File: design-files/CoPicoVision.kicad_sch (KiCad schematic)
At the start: 31 parts, among them J101 USB_C_Receptacle_PowerOnly_6P, Q101 MMFTP3334K-AQ, SW101 SW_Push, SW102 SW_Push, U101 Z80CPU, U102 DS1813, U103 74ACT05, U104 ICL7660A, U105 MAX16054, X101 3.579545MHZ

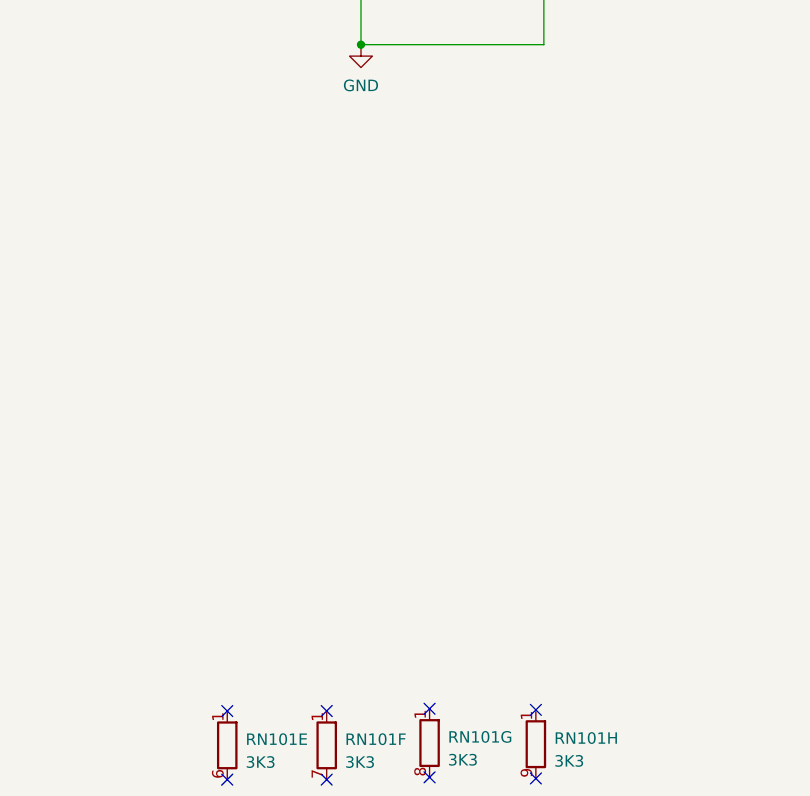
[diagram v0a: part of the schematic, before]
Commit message: Add cartridge connector.
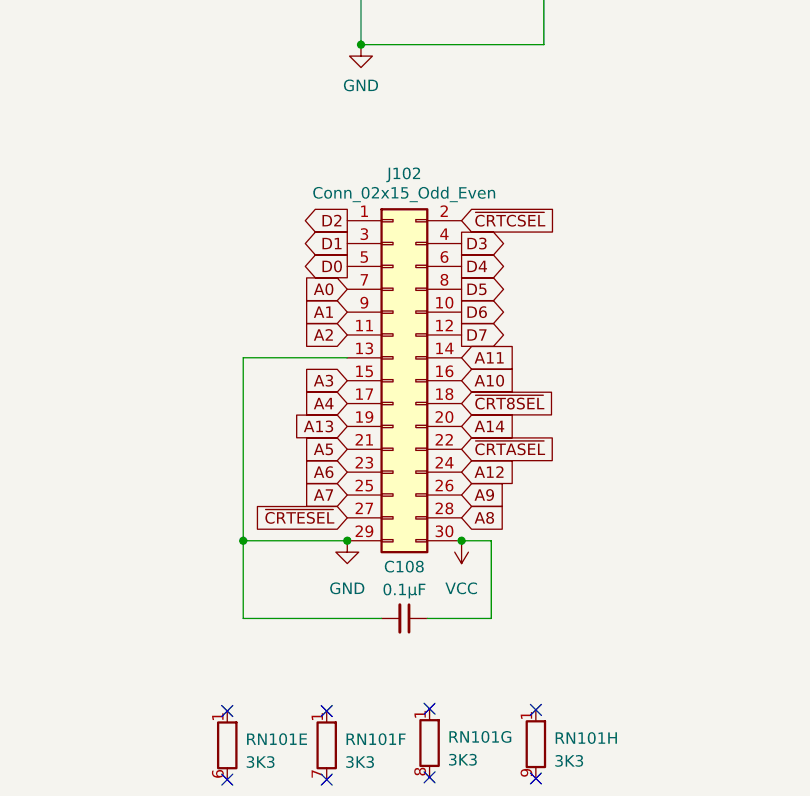
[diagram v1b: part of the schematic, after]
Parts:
- added C108: 0.1µF, Capacitor_SMD:C_0805_2012Metric_Pad1.18x1.45mm_HandSolder, symbol Device:C_Small
- added J102: Conn_02x15_Odd_Even, symbol Connector_Generic:Conn_02x15_Odd_Even
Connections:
- net A0: now also J102.7 (Pin_7)
- net A1: now also J102.9 (Pin_9)
- net A10: now also J102.16 (Pin_16)
- net A11: now also J102.14 (Pin_14)
- net A12: now also J102.24 (Pin_24)
- net A13: now also J102.19 (Pin_19)
- net A14: now also J102.20 (Pin_20)
- net A2: now also J102.11 (Pin_11)
- net A3: now also J102.15 (Pin_15)
- net A4: now also J102.17 (Pin_17)
- net A5: now also J102.21 (Pin_21)
- net A6: now also J102.23 (Pin_23)
- net A7: now also J102.25 (Pin_25)
- net A8: now also J102.28 (Pin_28)
- net A9: now also J102.26 (Pin_26)
- net D0: now also J102.5 (Pin_5)
- net D1: now also J102.3 (Pin_3)
- net D2: now also J102.1 (Pin_1)
- net D3: now also J102.4 (Pin_4)
- net D4: now also J102.6 (Pin_6)
- net D5: now also J102.8 (Pin_8)
- net D6: now also J102.10 (Pin_10)
- net D7: now also J102.12 (Pin_12)
- net GND: now also C108.2, J102.13 (Pin_13), J102.29 (Pin_29)
- net VCC: now also C108.1, J102.30 (Pin_30)
- new net ~{CRT8SEL}: J102.18 (Pin_18)
- new net ~{CRTASEL}: J102.22 (Pin_22)
- new net ~{CRTCSEL}: J102.2 (Pin_2)
- new net ~{CRTESEL}: J102.27 (Pin_27)

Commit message: Cartridge slot.
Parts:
- J102: footprint (none) -> jrt-Connectors:Sullins_Cart_Slot; Mouser (none) -> 571-5530843-2
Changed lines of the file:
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@@
       (effects (font (size 1.27 1.27)))
     )
-    (property "Footprint" "" (at 197.612 117.856 0)
+    (property "Footprint" "jrt-Connectors:Sullins_Cart_Slot" (at 197.612 117.856 0)
       (effects (font (size 1.27 1.27)) hide)
     )
-    (property "Datasheet" "~" (at 197.612 117.856 0)
+    (property "Datasheet" "https://www.te.com/commerce/DocumentDelivery/DDEController?Action=srchrtrv&DocNm=5530843&DocType=Customer+Drawing&DocLang=English&PartCntxt=5530843-2&DocFormat=pdf" (at 197.612 117.856 0)
       (effects (font (size 1.27 1.27)) hide)
     )
+    (property "Mouser" "571-5530843-2" (at 197.612 117.856 0)
+      (effects (font (size 1.27 1.27)) hide)
+    )
